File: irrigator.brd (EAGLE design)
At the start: 74.9 x 42.4 mm, 27 parts, among them IC1 MEGA8-AI, IC2 78L05Z, T1 BT136, X1 MSTBA2

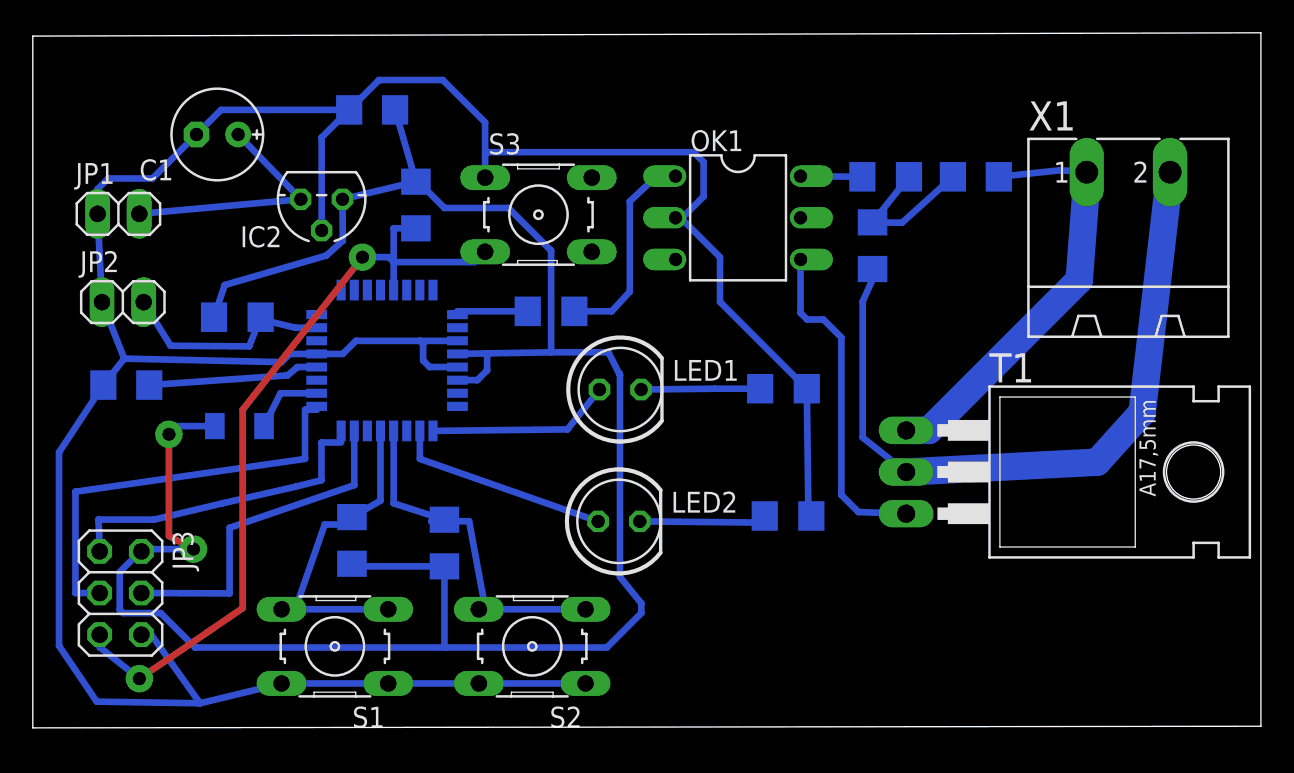
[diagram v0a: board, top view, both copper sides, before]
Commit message: fix. and topor files
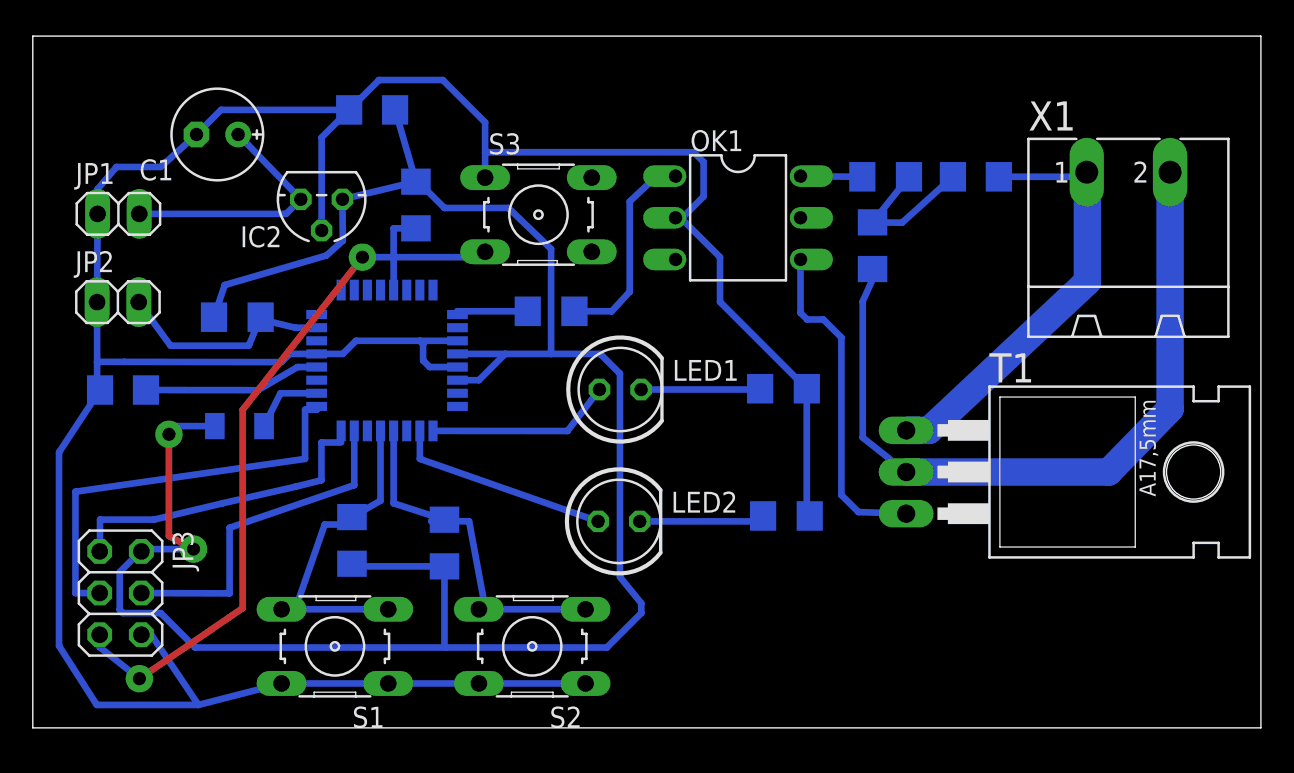
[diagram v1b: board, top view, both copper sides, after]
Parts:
- moved C4 0.36 mm to (5.50, 20.6)
- moved JP2 0.30 mm to (5.19, 26.0)
- moved R5 0.10 mm to (46.0, 12.9)
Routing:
- net N$7: track 44.4 -> 46.1 mm
- net GND: track 172.2 -> 173.4 mm
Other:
- board size 74.9 x 42.4 mm -> 74.9 x 42.2 mm
